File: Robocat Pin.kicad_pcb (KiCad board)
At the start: 2 copper layers, 62.9 x 62.9 mm, 20 parts, among them SW1 SW_DP3T, U1 NA555P

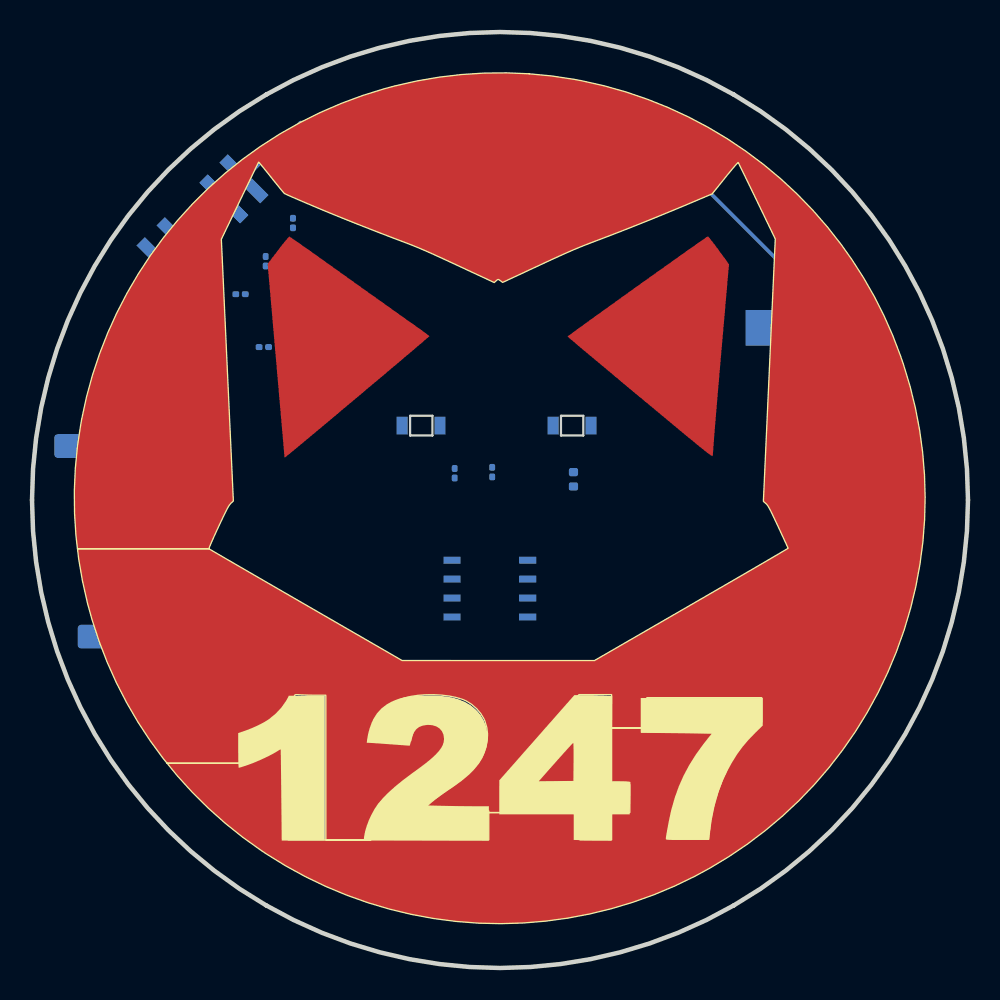
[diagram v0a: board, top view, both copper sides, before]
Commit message: Set all the traces
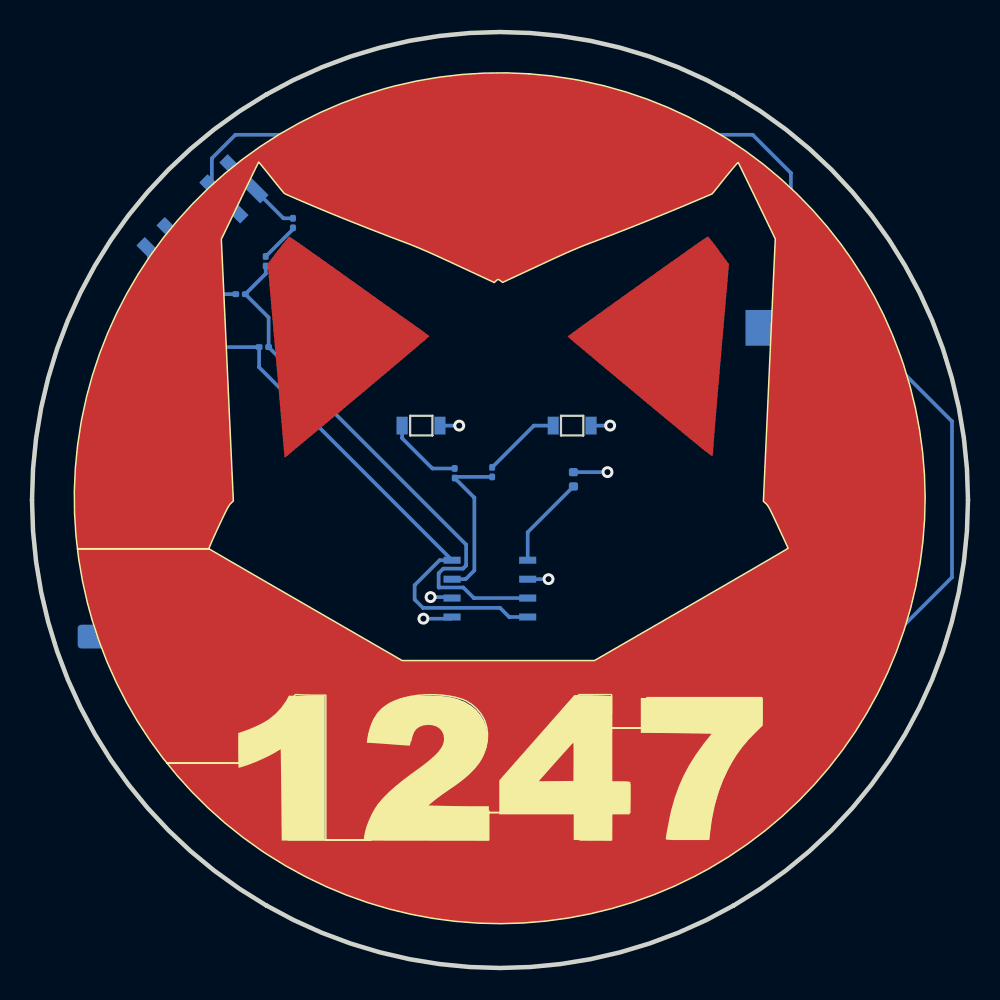
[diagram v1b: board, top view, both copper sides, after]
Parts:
- moved C4 2.77 mm to (30.3, 49.0)
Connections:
- net Net-(BT1-Pad1) renamed /gnd
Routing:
- net /gnd: track 0.00 -> 117.3 mm, vias 0 -> 10
- net Net-(C2-Pad1): track 0.00 -> 110.9 mm, vias 0 -> 8
- net Net-(R1-Pad1): track 0.00 -> 56.5 mm
- net Net-(BT1-Pad2): track 48.5 -> 90.5 mm
- net Net-(R1-Pad2): track 0.00 -> 36.1 mm
- net Net-(R5-Pad1): track 0.00 -> 11.0 mm
- net Net-(C1-Pad2): track 0.00 -> 6.23 mm
- net Net-(D2-Pad2): track 0.00 -> 5.26 mm
- net Net-(D1-Pad2): track 0.00 -> 5.22 mm
- net Net-(R4-Pad1): track 0.00 -> 4.78 mm
- net Net-(R3-Pad1): track 0.00 -> 3.25 mm
- net Net-(R2-Pad1): track 0.00 -> 2.71 mm
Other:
- copper layers 2 -> 4
